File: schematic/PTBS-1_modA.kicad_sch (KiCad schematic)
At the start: 149 parts, among them J1 MONO PHONE, J15 DC 2.1mm, J2 MONO PHONE, J3 MONO PHONE, J4 MONO PHONE, J5 MONO PHONE, J6 MONO PHONE, J7 MONO PHONE, J8 PHONE STEREO, J9 5pin, Q1 2SC1815Y, Q10 2SC1815Y, Q11 2SC1815Y, Q12 2SC1815Y, Q13 2SA1358, Q2 2SC1815Y, Q3 2SC1815, Q4 2SC1815Y, Q5 2SC1815Y, Q6 2SC1815Y, Q7 2SK660, Q8 2SA1015Y, Q9 2SC1815Y, SW1 SW_Push, SW10 SW_SPST, SW2 SW_Push, SW3 SW_Push, SW4 SW_Push, SW5 SW_Push, SW6 SW_Push, SW7 SW_Push, SW8 SW_Push, SW9 SW_DPST, U1 L7805, U2 PIC16F873A, U3 NAR161H-F, X1 10.0MT

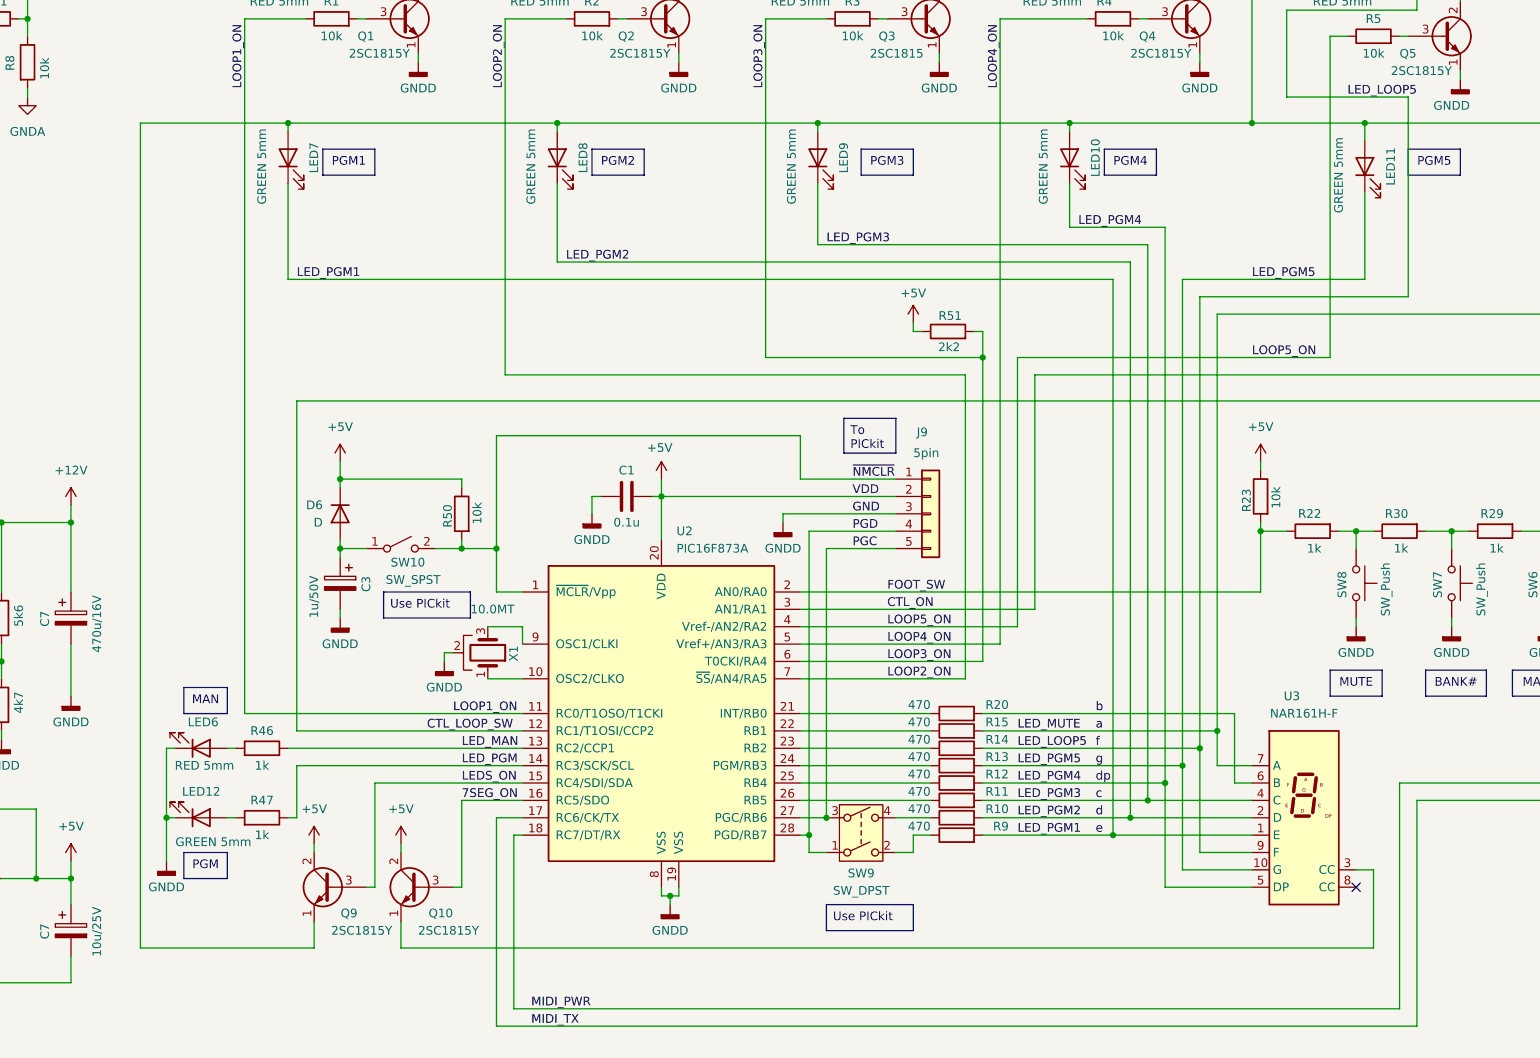
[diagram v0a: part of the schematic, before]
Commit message: Update PTBS-1_modA.kicad_sch
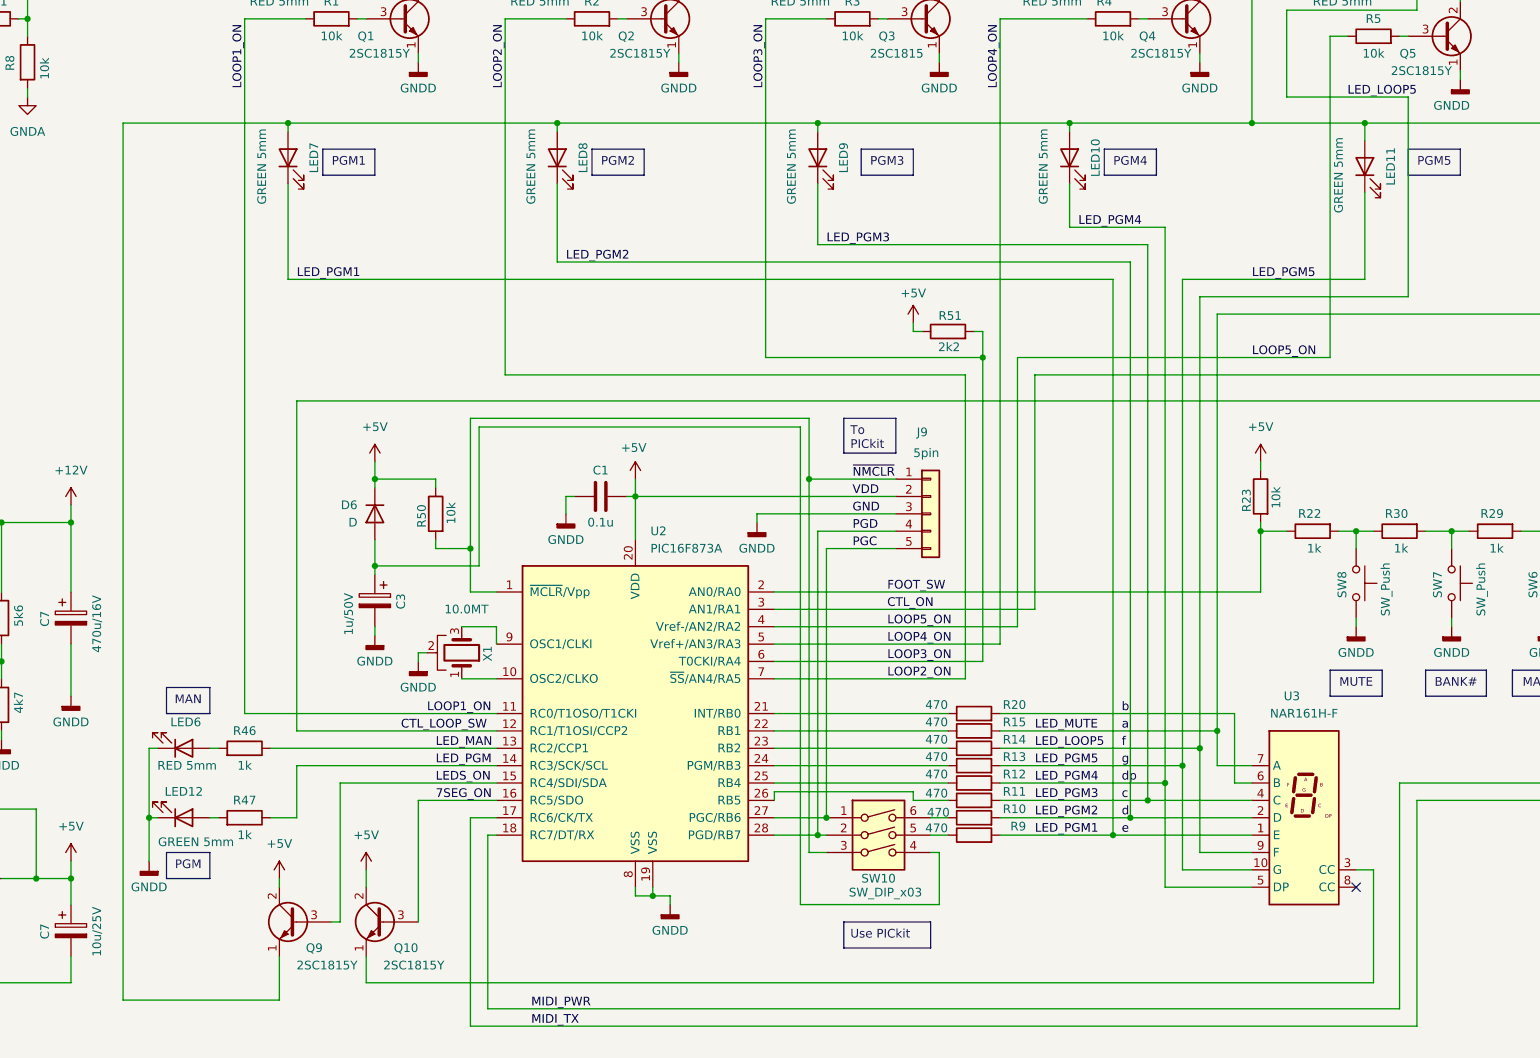
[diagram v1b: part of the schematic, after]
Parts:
- removed SW10: SW_SPST, symbol Switch:SW_SPST
- removed SW9: SW_DPST, symbol Switch:SW_DPST
- added SW10: SW_DIP_x03, symbol Switch:SW_DIP_x03
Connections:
- net PGC: now also SW10.1
- net PGD: now also SW10.2
- net ~{NMCLR}: now also SW10.3
- net at R9.1: now also SW10.5
- net at C3.1, D6.2 (A): now also SW10.4
- net at R10.1: now also SW10.6
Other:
- moved on the sheet: C1, C3, D6, LED12, LED6, Q10, Q9, R10, R11, R12, R13, R14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
